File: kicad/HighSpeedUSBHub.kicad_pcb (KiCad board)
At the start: 4 copper layers, 80.6 x 49 mm, 86 parts, among them U1 TUSB8041IRGCR, U2 TPS2561DRCR, U4 TPS2561DRCR, U5 SY8089A1AAC, U6 XC6206P332MR_C5148692, X1 X322524MRB4SI

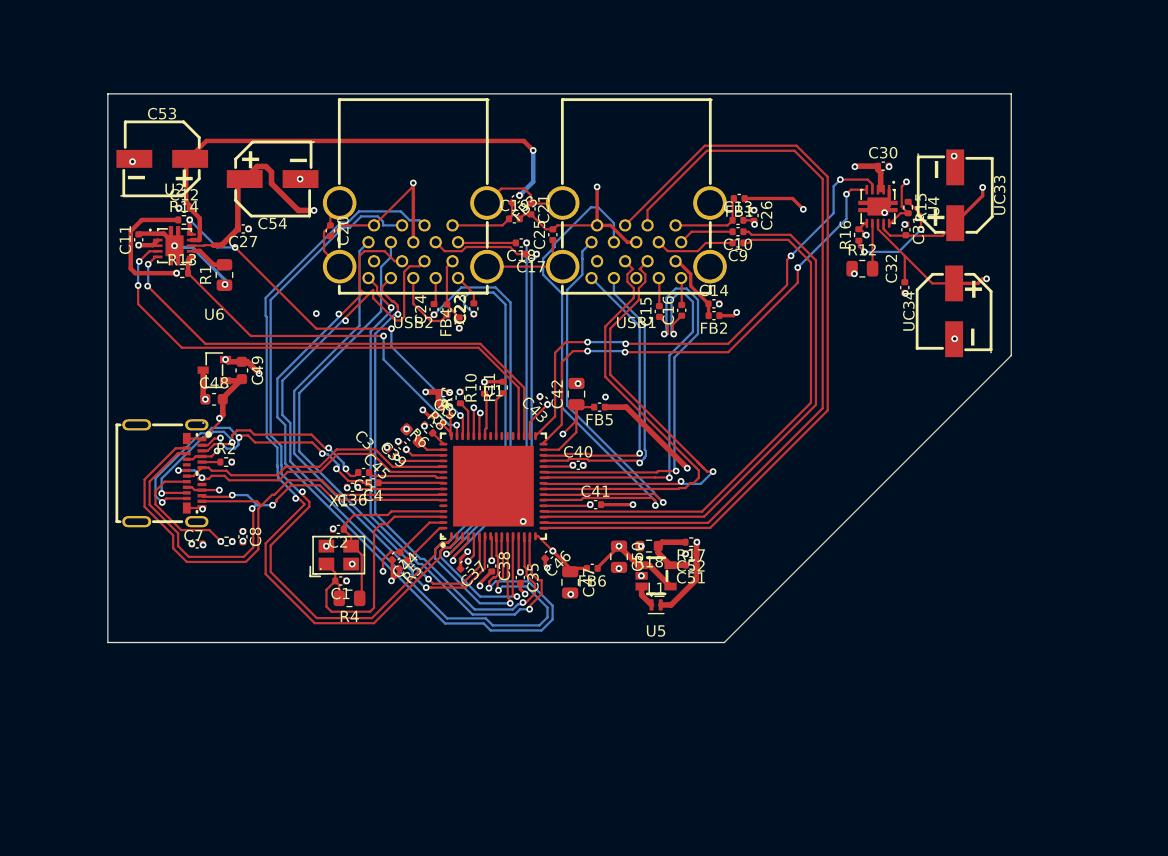
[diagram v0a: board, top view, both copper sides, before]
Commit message: upload
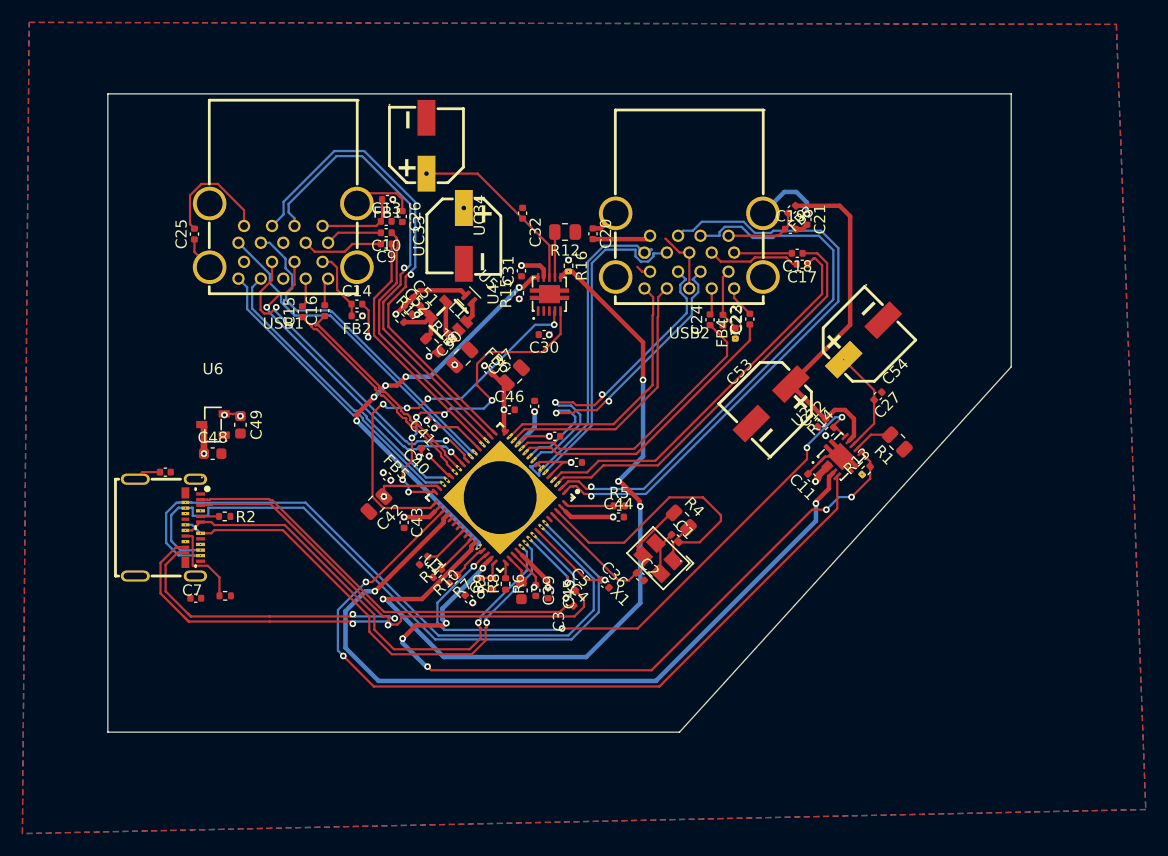
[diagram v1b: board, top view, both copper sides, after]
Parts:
- moved C11 63.7 mm to (130.7, 142.0), turned to 135 degrees
- moved R13 63.5 mm to (135.6, 141.4), turned to 45 degrees
- moved U2 62.4 mm to (133.4, 140.2), turned to 45 degrees
- moved R1 61.8 mm to (138.4, 138.9), turned to 135 degrees
- moved R14 60.6 mm to (132.4, 137.9), turned to 45 degrees
- moved C12 60.0 mm to (131.6, 137.2), turned to 45 degrees
- moved C27 58.6 mm to (136.7, 134.8), turned to -135 degrees
- moved C53 58.6 mm to (127.1, 135.4), turned to 45 degrees
- moved C54 54.6 mm to (135.4, 129.8), turned to -135 degrees
- moved UC34 49.3 mm to (96.4, 112.4), turned to -90 degrees
- moved UC33 44.0 mm to (99.7, 120.5), turned to 90 degrees
- moved R15 35.5 mm to (104.6, 125.6), turned to 90 degrees
- moved C32 34.7 mm to (104.9, 118.4), turned to -90 degrees
- moved C31 34.5 mm to (104.8, 123.6), turned to 90 degrees
- moved C51 34.0 mm to (95.5, 126.4), turned to -45 degrees
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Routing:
- net GND: track 85.2 -> 40.7 mm, vias 51 -> 5
- net /USB2_D-: track 70.4 -> 28.3 mm
- net /USB2_D+: track 70.4 -> 28.9 mm
- net /USB_C_SSTX-: track 29.3 -> 69.5 mm, vias 4 -> 2
- net BOARD_3P3V: track 121.4 -> 87.0 mm, vias 6 -> 8
- net /OVERCUR2Z: track 33.4 -> 65.0 mm, vias 2 -> 6
- net /USB_C_SSTX+: track 33.7 -> 64.3 mm, vias 5 -> 2
- net /USB3_D+: track 72.7 -> 43.7 mm, vias 0 -> 1
- net /OVERCUR4Z: track 45.0 -> 72.8 mm, vias 2 -> 4
- net /USB3_D-: track 69.8 -> 42.4 mm, vias 0 -> 1
- net /PWRCTL2_BATEN2: track 44.8 -> 72.0 mm
- net /USB3_SSTX+: track 48.9 -> 23.4 mm
- net /USB3_SSTX-: track 47.4 -> 22.5 mm
- net /USB2_SSRX-: track 48.4 -> 23.6 mm, vias 2 -> 0
- net /PWRCTL1_BATEN1: track 47.2 -> 70.2 mm
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- added copper zone on B.Cu, net GND
- added copper zone on F.Cu, net GND
- added copper zone on In2.Cu, net GND
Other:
- board size 80.6 x 49 mm -> 80.6 x 57 mm
